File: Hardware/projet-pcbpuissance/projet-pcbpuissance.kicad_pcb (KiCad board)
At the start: 2 copper layers, 52.4 x 45.8 mm, 35 parts, among them J2 Conn_01x02, J3 Conn_01x02, J4 Conn_01x02, U1 MAX5033DUSA+, U2 MAX5033DUSA+

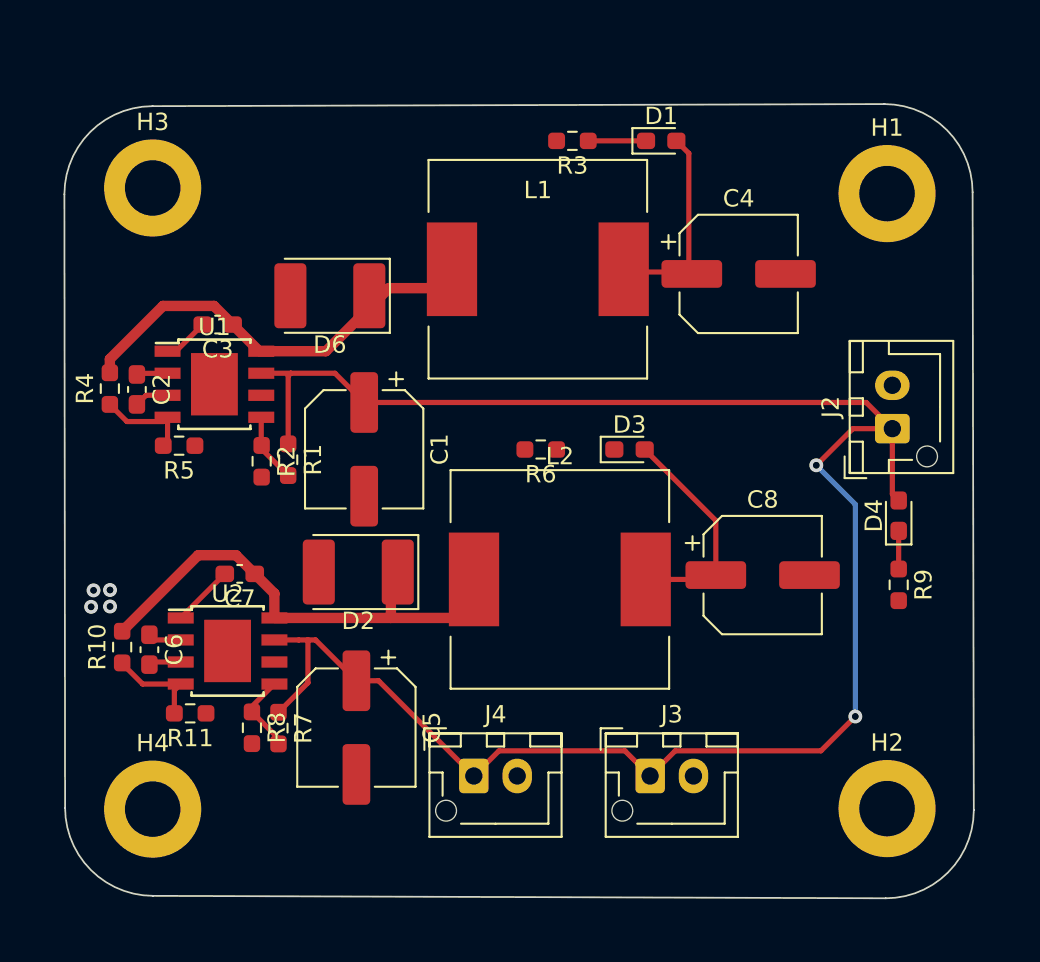
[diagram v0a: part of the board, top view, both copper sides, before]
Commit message: Modif PCB
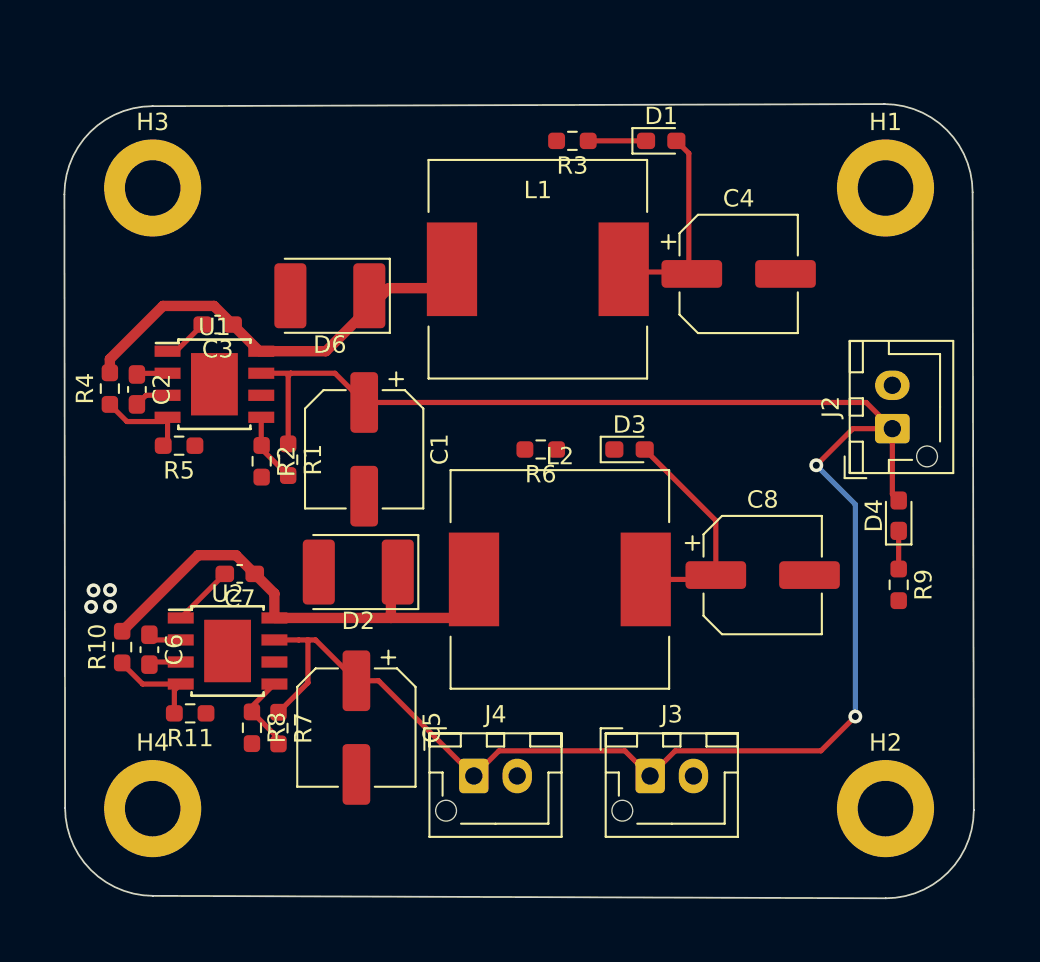
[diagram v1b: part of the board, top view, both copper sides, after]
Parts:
- moved H1 0.34 mm to (142.7, 72.7)
- moved H2 0.09 mm to (142.7, 108.5)
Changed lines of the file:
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@@
   )
   (footprint "MountingHole:MountingHole_3.2mm_M3_DIN965_Pad" (layer "F.Cu")
-    (at 142.8125 108.45)
+    (at 142.7225 108.45)
     (descr "Mounting Hole 3.2mm, M3, DIN965")
     (tags "mounting hole 3.2mm m3 din965")
@@
   )
   (footprint "MountingHole:MountingHole_3.2mm_M3_DIN965_Pad" (layer "F.Cu")
-    (at 100.4805 108.48)
+    (at 100.4805 108.45)
     (descr "Mounting Hole 3.2mm, M3, DIN965")
     (tags "mounting hole 3.2mm m3 din965")
@@
   )
   (footprint "MountingHole:MountingHole_3.2mm_M3_DIN965_Pad" (layer "F.Cu")
-    (at 142.8125 73)
+    (at 142.7225 72.676)
     (descr "Mounting Hole 3.2mm, M3, DIN965")
     (tags "mounting hole 3.2mm m3 din965")
